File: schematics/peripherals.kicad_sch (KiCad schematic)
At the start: 4 parts

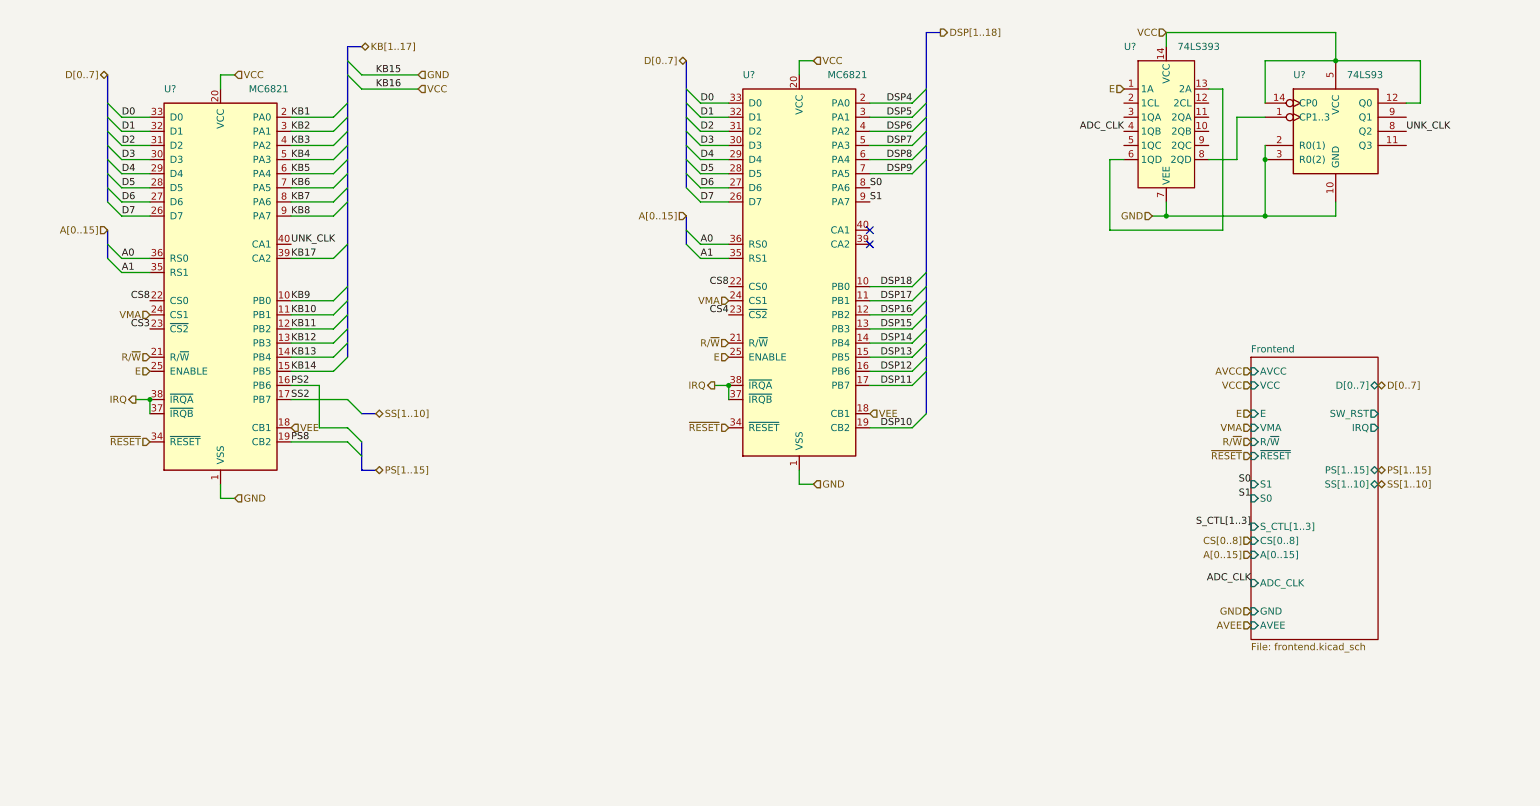
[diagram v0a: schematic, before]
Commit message: cleanup, fixes, started on power supplies
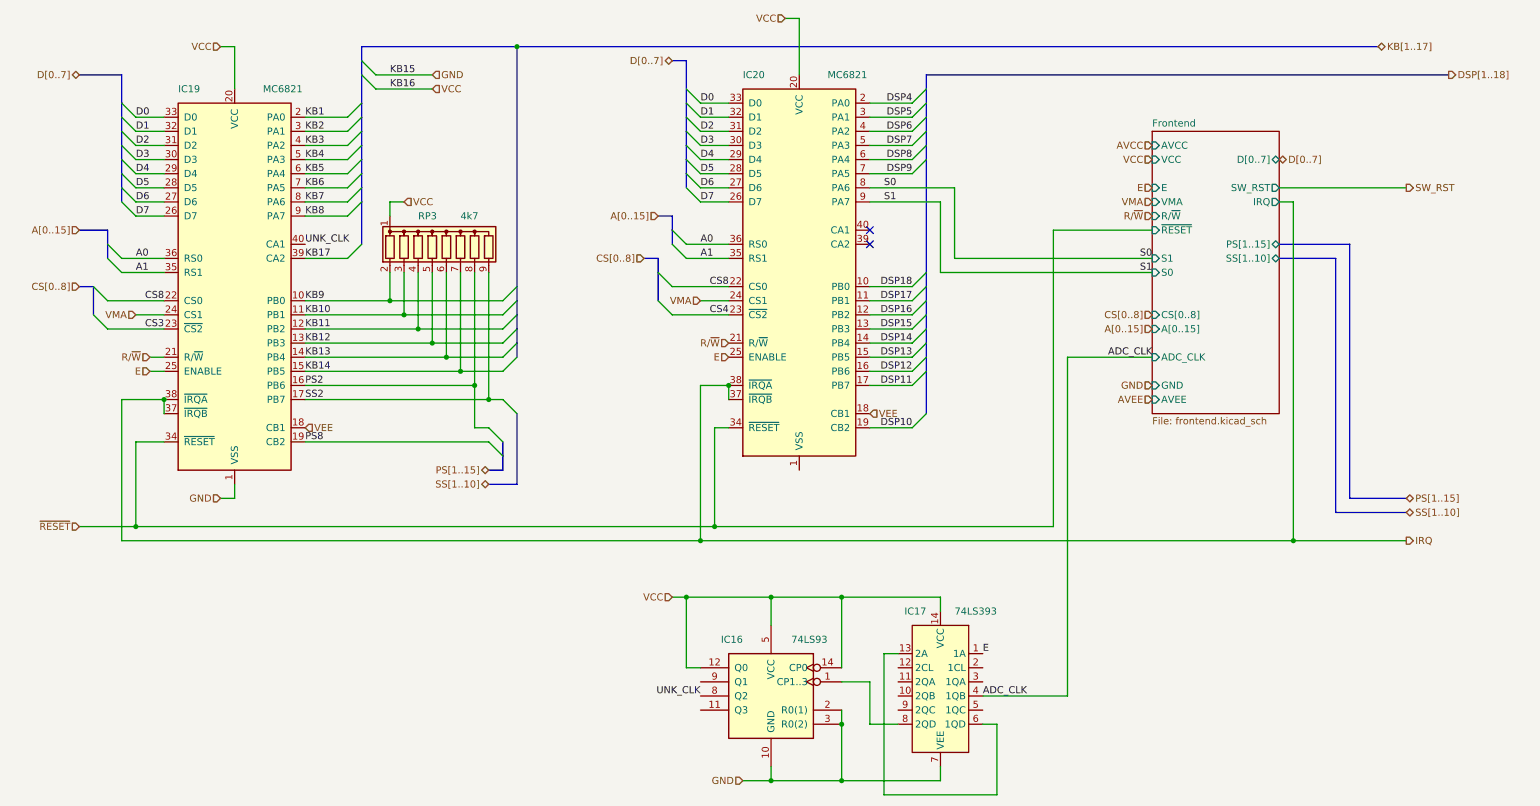
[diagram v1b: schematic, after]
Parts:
- added RP3: 4k7, Resistor_THT:R_Array_SIP9, symbol Device:R_Network08
- IC19, IC20: renamed from U?; footprint (none) -> Package_DIP:DIP-40_W15.24mm
- gave numbers to parts that had none: 2
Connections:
- net GND: no longer IC20.1 (VSS)
- net KB10: now also RP3.3 (R2)
- net KB11: now also RP3.4 (R3)
- net KB12: now also RP3.5 (R4)
- net KB13: now also RP3.6 (R5)
- net KB14: now also RP3.7 (R6)
- net KB9: now also RP3.2 (R1)
- net PS2: now also RP3.8 (R7)
- net SS2: now also RP3.9 (R8)
- net VCC: now also RP3.1 (common)
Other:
- sheet Frontend ports: added none; removed S_CTL[1..3]
- moved on the sheet: IC16, IC17, IC19
